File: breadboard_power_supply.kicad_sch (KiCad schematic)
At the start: 0 parts

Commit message: Added schematic for usb-c input and variable voltage outputmax. 500mA 0.55V-5V
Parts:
- added C1, C2: C, symbol Device:C
- added D1: D_Schottky, symbol Device:D_Schottky
- added J1: USB_C_Receptacle_USB2.0_16P, symbol Connector:USB_C_Receptacle_USB2.0_16P
- added J2: Conn_01x02_Pin, symbol Connector:Conn_01x02_Pin
- added R1, R2: 5k1, symbol Device:R
- added R3: R_Variable, symbol Device:R_Variable
- added R5, R6, R7, R8: R, symbol Device:R
- added SW1: SW_SP3T, symbol Switch:SW_SP3T
- added SW2: SW_SPST, symbol Switch:SW_SPST
- added U1: TLV75801PDRV, Package_SON:WSON-6-1EP_2x2mm_P0.65mm_EP1x1.6mm, symbol Regulator_Linear:TLV75801PDRV
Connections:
- new net: C1.2, D1.1 (K), J1.A4 (VBUS), J1.A9 (VBUS), J1.B4 (VBUS), J1.B9 (VBUS), SW2.1 (A), U1.6 (IN)
- new net: J1.A5 (CC1), R1.1
- new net: J1.B5 (CC2), R2.1
- new net: R8.1, SW1.2
- new net: R6.1, SW2.2 (B), U1.4 (EN)
- new net: C2.1, D1.2 (A), J2.2 (Pin_2), R5.1, U1.1 (OUT)
- new net: R3.1, SW1.1
- new net: R5.2, SW1.3, U1.2 (FB)
- new net: R7.1, SW1.4
- new net GND: C1.1, C2.2, J1.A1 (GND), J1.A12 (GND), J1.B1 (GND), J1.B12 (GND), J1.SH (SHIELD), J2.1 (Pin_1), R1.2, R2.2, R3.2, R6.2, R7.2, R8.2, U1.3 (GND), U1.7 (GND)
- no-connect marks 0 -> 6

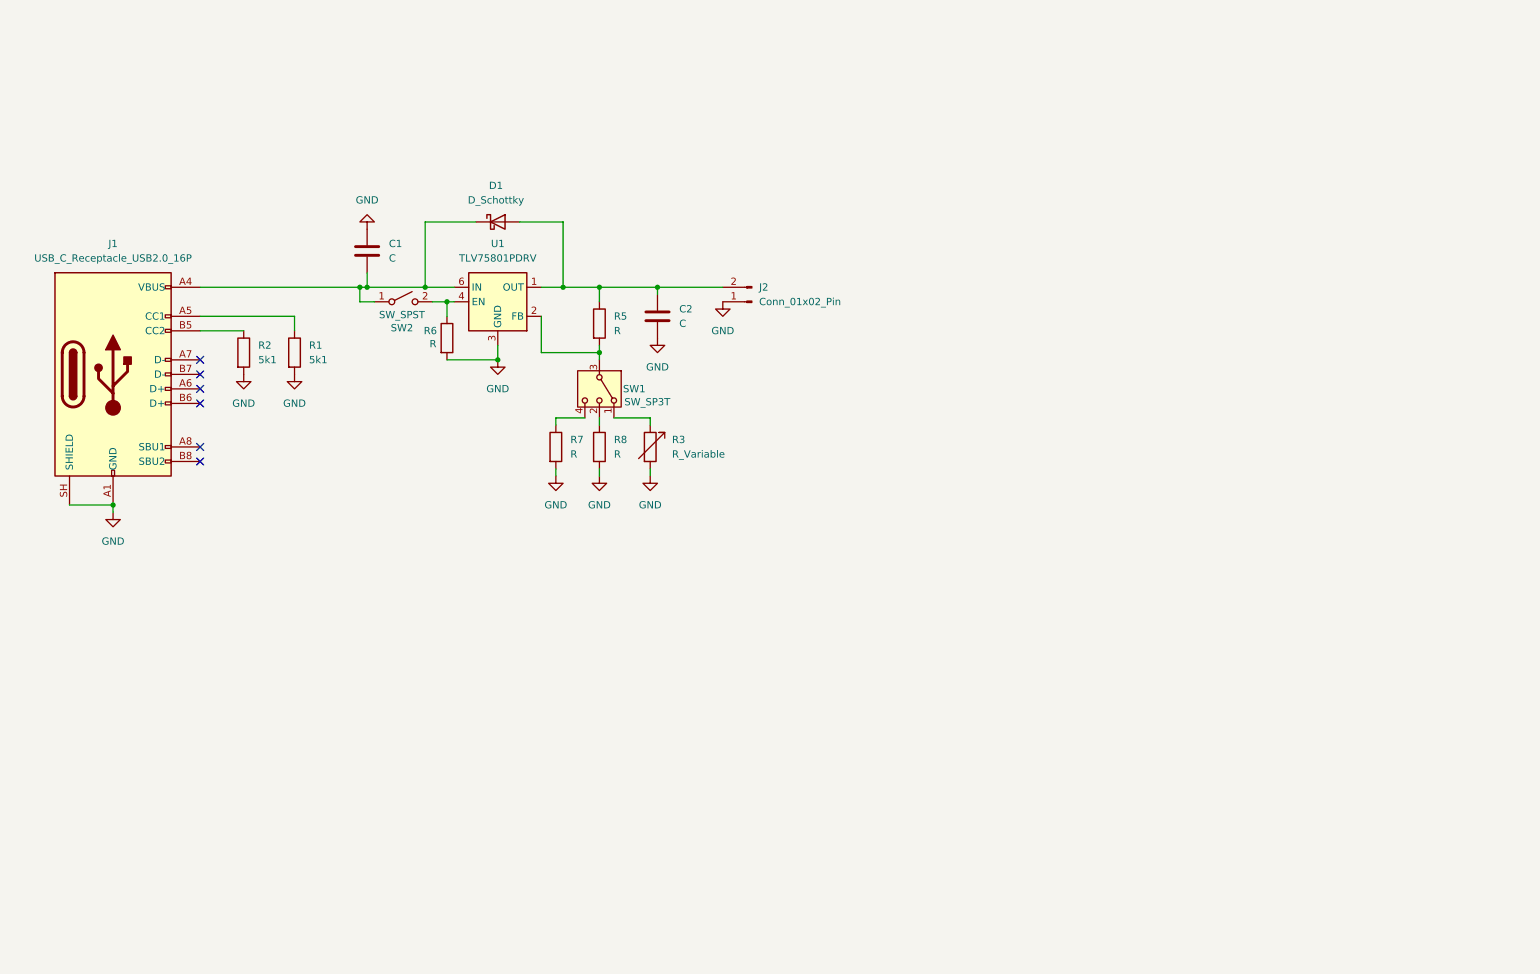
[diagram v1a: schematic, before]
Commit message: Added second voltage output and annotations
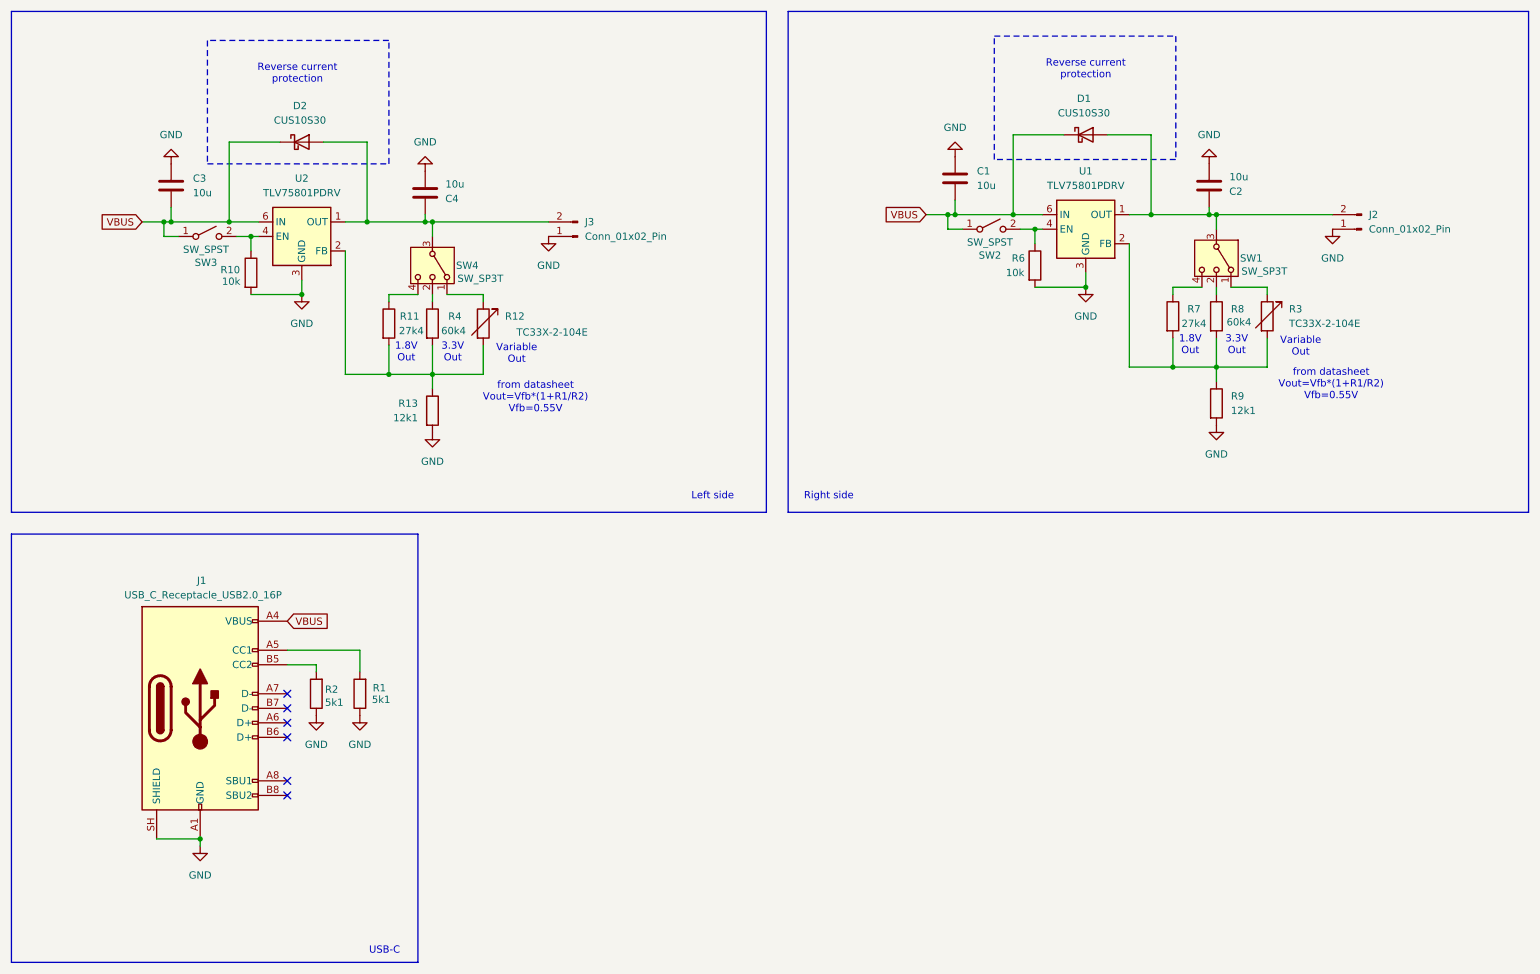
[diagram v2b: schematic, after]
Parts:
- removed R5: R, symbol Device:R
- added C3, C4: 10u, symbol Device:C
- added D2: CUS10S30, symbol Device:D_Schottky
- added J3: Conn_01x02_Pin, symbol Connector:Conn_01x02_Pin
- added R10: 10k, symbol Device:R
- added R11: 27k4, symbol Device:R
- added R12: 60k4, symbol Device:R
- added R13, R9: 12k1, symbol Device:R
- added R4: TC33X-2-104E, symbol Device:R_Variable
- added SW3: SW_SPST, symbol Switch:SW_SPST
- added SW4: SW_SP3T, symbol Switch:SW_SP3T
- added U2: TLV75801PDRV, Package_SON:WSON-6-1EP_2x2mm_P0.65mm_EP1x1.6mm, symbol Regulator_Linear:TLV75801PDRV
- C1, C2: value C -> 10u
- D1: value D_Schottky -> CUS10S30
- R3: value R_Variable -> TC33X-2-104E
- R6: value R -> 10k
- R7: value R -> 27k4
- R8: value R -> 60k4
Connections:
- net GND: now also R1.1, R2.1, C3.1, C4.2, J3.1 (Pin_1), R10.2, R13.2, R9.2, U2.3 (GND), U2.7 (GND); no longer R1.2, R2.2, R3.2, R7.2, R8.2
- net VBUS: now reaches C1.2, D1.1 (K), J1.A4 (VBUS), J1.A9 (VBUS), J1.B4 (VBUS), J1.B9 (VBUS), SW2.1 (A), U1.6 (IN)
- net VBUS: now also C3.2, D2.1 (K), SW3.1 (A), U2.6 (IN)
- net at J1.A5 (CC1): now also R1.2; no longer R1.1
- net at J1.B5 (CC2): now also R2.2; no longer R2.1
- net at C2.1, D1.2 (A), J2.2 (Pin_2)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: now also SW1.3
- net at U1.2 (FB): now also R3.2, R7.2, R8.2, R9.1; no longer SW1.3
- new net: R4.1, SW4.1
- new net: R11.2, R12.2, R13.1, R4.2, U2.2 (FB)
- new net: C4.1, D2.2 (A), J3.2 (Pin_2), SW4.3, U2.1 (OUT)
- new net: R10.1, SW3.2 (B), U2.4 (EN)
- new net: R12.1, SW4.2
- new net: R11.1, SW4.4
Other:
- note added: "1.8V Out"
- note added: "3.3V Out"
- note added: "Left side"
- note added: "Reverse current protection"
- note added: "Right side"
- note added: "USB-C"
- note added: "Variable Out"
- note added: "from datasheet Vout=Vfb*(1+R1/R2) Vfb=0.55V"
- moved on the sheet: C1, C2, D1, J1, J2, R1, R2, R3, R6, R7, R8, SW1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

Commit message: Made PCB layout
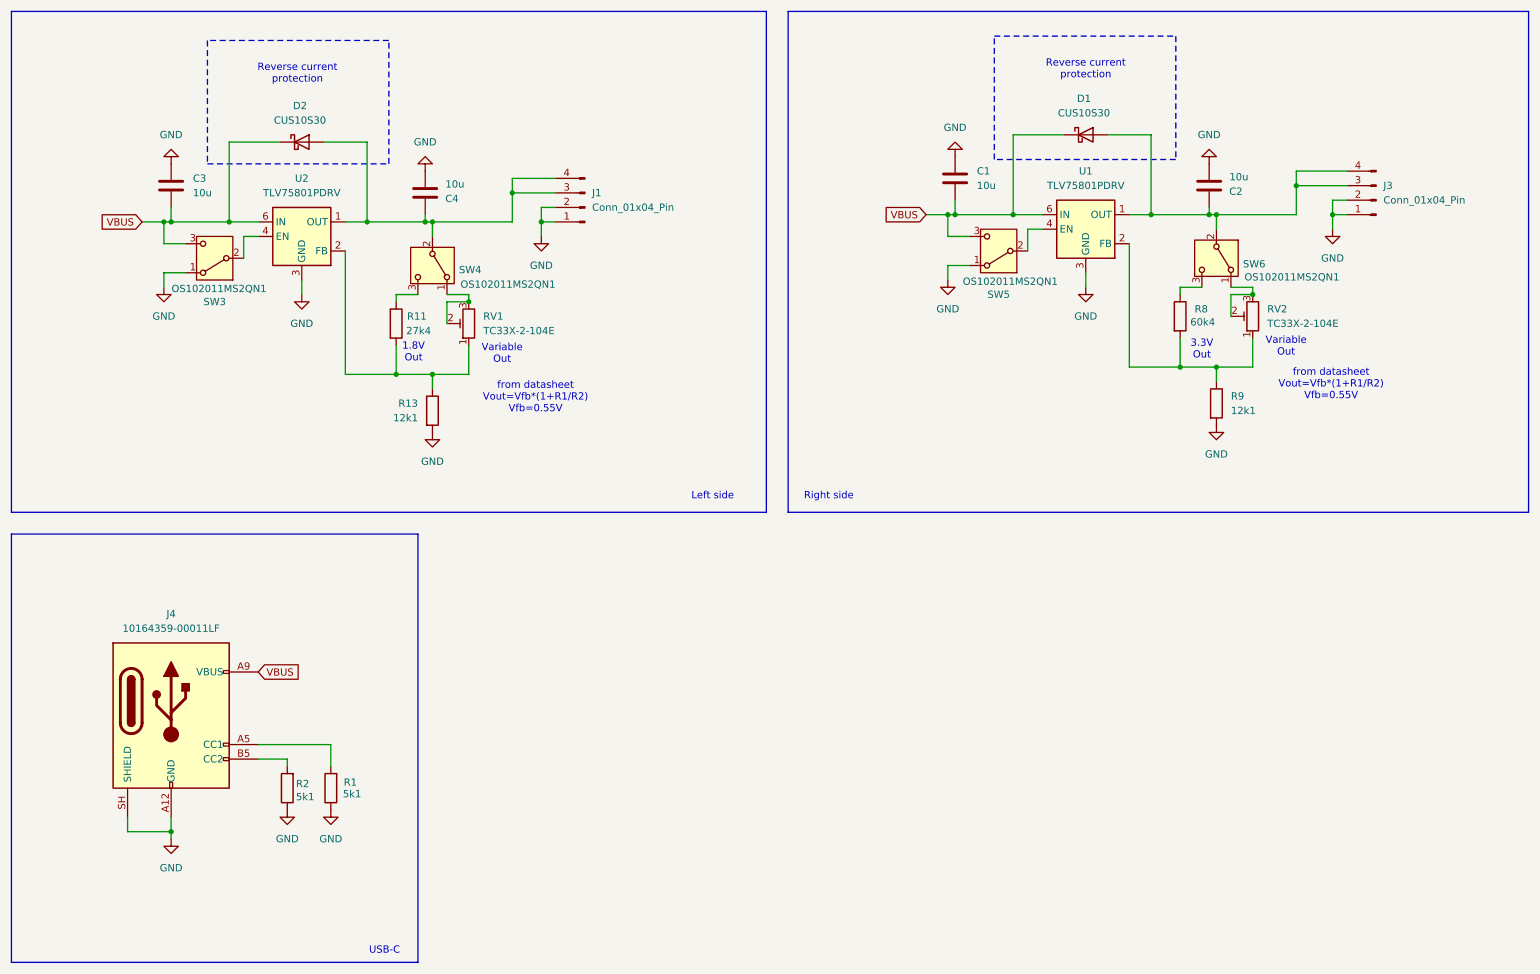
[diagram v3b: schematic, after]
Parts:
- removed J1: USB_C_Receptacle_USB2.0_16P, symbol Connector:USB_C_Receptacle_USB2.0_16P
- removed J2, J3: Conn_01x02_Pin, symbol Connector:Conn_01x02_Pin
- removed R10, R6: 10k, symbol Device:R
- removed R12: 60k4, symbol Device:R
- removed R3, R4: TC33X-2-104E, symbol Device:R_Variable
- removed R7: 27k4, symbol Device:R
- removed SW1, SW4: SW_SP3T, symbol Switch:SW_SP3T
- removed SW2, SW3: SW_SPST, symbol Switch:SW_SPST
- added J1, J3: Conn_01x04_Pin, Connector_PinHeader_2.54mm:PinHeader_2x02_P2.54mm_Vertical, symbol Connector:Conn_01x04_Pin
- added J4: 10164359-00011LF, local:AMPHENOL_10164359-00011LF, symbol Connector:USB_C_Receptacle_PowerOnly_6P
- added RV1, RV2: TC33X-2-104E, Potentiometer_SMD:Potentiometer_Bourns_TC33X_Vertical, symbol Device:R_Potentiometer_Trim
- added SW3, SW4, SW5, SW6: OS102011MS2QN1, local:SPDT_OS102011_CNK, symbol Switch:SW_SPDT
- C1, C2, C3, C4: footprint (none) -> Capacitor_SMD:C_0805_2012Metric_Pad1.18x1.45mm_HandSolder
- D1, D2: footprint (none) -> local:USC_TOS
- R1, R11, R13, R2, R8, R9: footprint (none) -> Resistor_SMD:R_0402_1005Metric_Pad0.72x0.64mm_HandSolder
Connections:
- net GND: now also J1.1 (Pin_1), J1.2 (Pin_2), J3.1 (Pin_1), J3.2 (Pin_2), J4.A12 (GND), J4.B12 (GND), J4.SH (SHIELD), SW3.1 (A), SW5.1 (A)
- net VBUS: now also J4.A9 (VBUS), J4.B9 (VBUS), SW3.3 (C), SW5.3 (C)
- net at R1.2: now also J4.A5 (CC1)
- net at R2.2: now also J4.B5 (CC2)
- net at R11.2, R13.1, U2.2 (FB): now also RV1.1
- net at C4.1, D2.2 (A), U2.1 (OUT): now also J1.3 (Pin_3), J1.4 (Pin_4), SW4.2 (B)
- net at U2.4 (EN): now also SW3.2 (B)
- net at R8.1: now also SW6.3 (C)
- net at R8.2, R9.1, U1.2 (FB): now also RV2.1
- net at U1.4 (EN): now also SW5.2 (B)
- net at C2.1, D1.2 (A), U1.1 (OUT): now also J3.3 (Pin_3), J3.4 (Pin_4), SW6.2 (B)
- net at R11.1: now also SW4.3 (C)
- new net: RV2.2, RV2.3, SW6.1 (A)
- new net: RV1.2, RV1.3, SW4.1 (A)
- no-connect marks 6 -> 0
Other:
- moved on the sheet: R1, R11, R2, R8
